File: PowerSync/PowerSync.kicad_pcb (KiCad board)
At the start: 2 copper layers, 107.3 x 48.9 mm, 40 parts, among them K12VDC1 G5RL-K1A-E, K9VAC1 G5RL-K1A-E, Q1 2N3904, Q2 2N3904, U1 74HCT1G04, U2 74HCT1G32, U3 74HCT74, U4 74HCT2G08

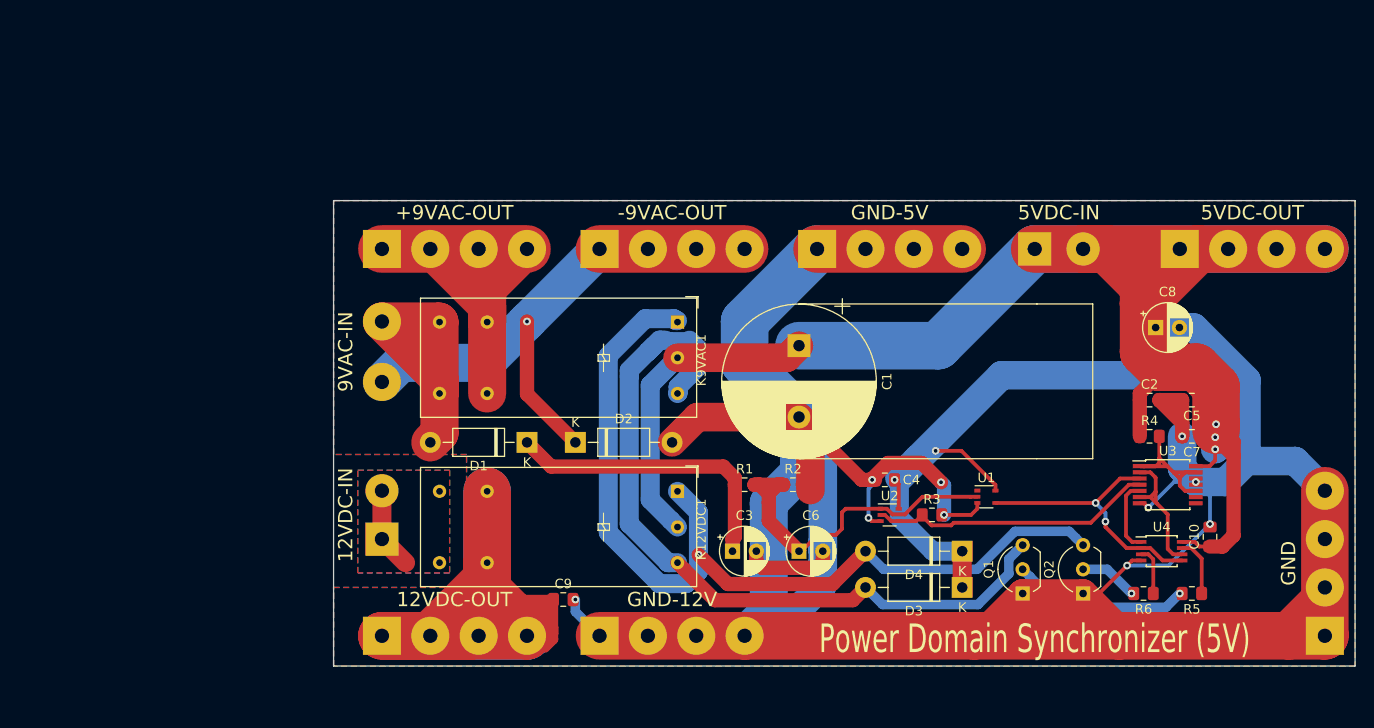
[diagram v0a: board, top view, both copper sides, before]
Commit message: Add files via upload
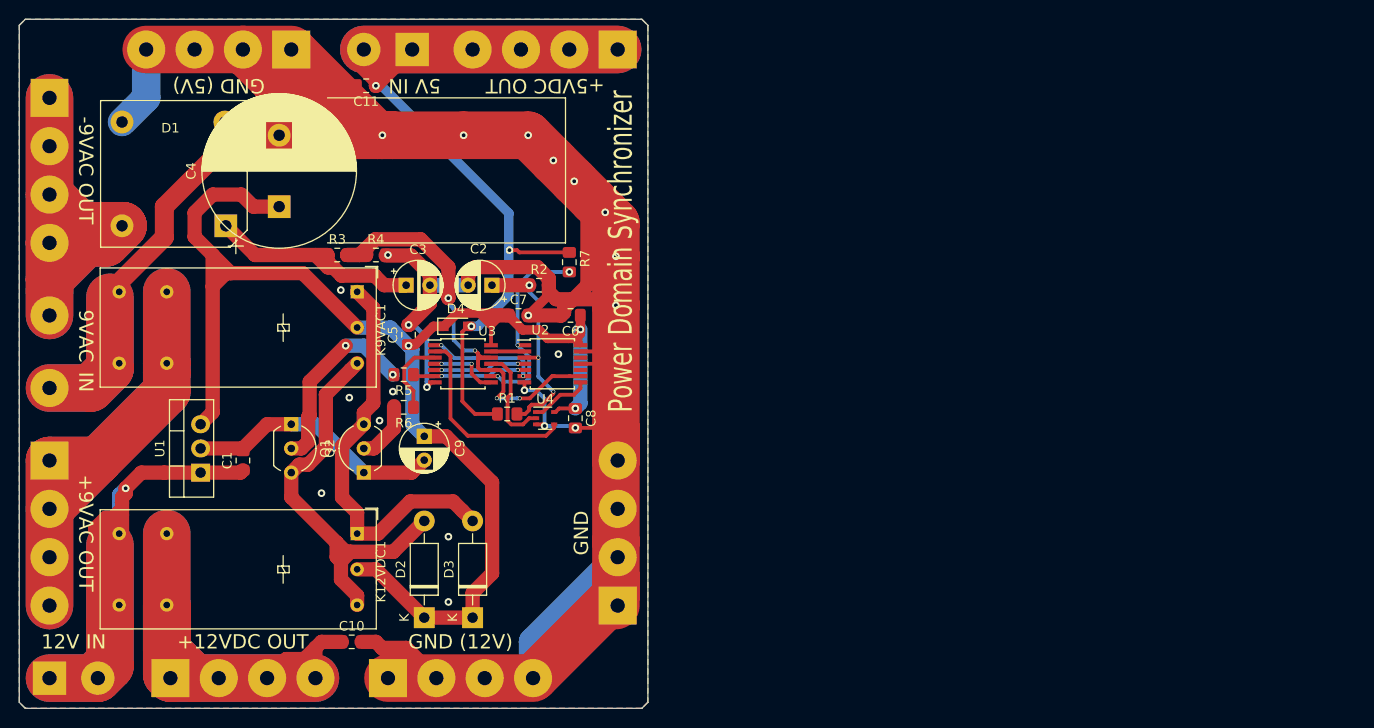
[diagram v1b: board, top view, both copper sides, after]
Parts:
- removed +9VAC-OUT, -9VAC-OUT, 12VDC-OUT, 5VDC-OUT, GND-12V: ~, Connector_Wire:SolderWirePad_1x04_P5.08mm_Drill1.5mm
- removed 12VDC-IN: +12VDC, Connector_Wire:SolderWirePad_1x02_P5.08mm_Drill1.5mm
- removed 5VDC-IN: +5VDC, Connector_Wire:SolderWirePad_1x02_P5.08mm_Drill1.5mm
- removed 9VAC-IN: +9VAC, Connector_Wire:SolderWirePad_1x01_Drill1.5mm
- removed GND-5V: GND, Connector_Wire:SolderWirePad_1x04_P5.08mm_Drill1.5mm
- removed IN-2: -9VAC, Connector_Wire:SolderWirePad_1x01_Drill1.5mm
- removed the REF** at (142.4, 83.1)
- added +12VDC OUT: ~, Connector_Wire:SolderWirePad_1x04_P5.08mm_Drill1.5mm, F.Cu at (58.4, 109.2)
- added +5VDC OUT: ~, Connector_Wire:SolderWirePad_1x04_P5.08mm_Drill1.5mm, F.Cu at (105.4, 43.2)
- added +9VAC OUT: ~, Connector_Wire:SolderWirePad_1x04_P5.08mm_Drill1.5mm, F.Cu at (45.7, 86.4)
- added -9VAC OUT: ~, Connector_Wire:SolderWirePad_1x04_P5.08mm_Drill1.5mm, F.Cu at (45.7, 48.3)
- added 12V IN: +12VDC, Connector_Wire:SolderWirePad_1x02_P5.08mm_Drill1.5mm, F.Cu at (45.7, 109.2)
- added 5V IN: +5VDC, Connector_Wire:SolderWirePad_1x02_P5.08mm_Drill1.5mm, F.Cu at (83.8, 43.2)
- added 9VAC: -9VAC, Connector_Wire:SolderWirePad_1x01_Drill1.5mm, F.Cu at (45.7, 71.1)
- added C11: 100n, Capacitor_SMD:C_0805_2012Metric_Pad1.15x1.40mm_HandSolder, F.Cu at (79.0, 47.0)
- added GND (12V): ~, Connector_Wire:SolderWirePad_1x04_P5.08mm_Drill1.5mm, F.Cu at (81.3, 109.2)
- added GND (5V): GND, Connector_Wire:SolderWirePad_1x04_P5.08mm_Drill1.5mm, F.Cu at (71.1, 43.2)
- added IN: +9VAC, Connector_Wire:SolderWirePad_1x01_Drill1.5mm, F.Cu at (45.7, 78.7)
- added R7: 220, Resistor_SMD:R_0805_2012Metric_Pad1.15x1.40mm_HandSolder, F.Cu at (100.3, 65.5)
- added REF**: OSHW-Logo_19x20mm_SilkScreen, Symbol:OSHW-Logo_19x20mm_SilkScreen, B.Cu at (92.8, 57.0)
- C1: value 10000u -> 220n; footprint Capacitor_THT:CP_Radial_D16.0mm_P7.50mm -> Capacitor_SMD:C_0805_2012Metric_Pad1.15x1.40mm_HandSolder
- C2: value 220n -> 1u; footprint Capacitor_SMD:C_0805_2012Metric_Pad1.15x1.40mm_HandSolder -> Capacitor_THT:CP_Radial_D5.0mm_P2.50mm
- C4: value 100n -> 10000u; footprint Capacitor_SMD:C_0805_2012Metric_Pad1.15x1.40mm_HandSolder -> Capacitor_THT:CP_Radial_D16.0mm_P7.50mm
- C5: value 47n -> 220n
- C6: value 2u2 -> 100n; footprint Capacitor_THT:CP_Radial_D5.0mm_P2.50mm -> Capacitor_SMD:C_0805_2012Metric_Pad1.15x1.40mm_HandSolder
- C7: value 10n -> 47n
- C8: value 10u -> 10n; footprint Capacitor_THT:CP_Radial_D5.0mm_P2.50mm -> Capacitor_SMD:C_0805_2012Metric_Pad1.15x1.40mm_HandSolder
- C9: value 100n -> 10u; footprint Capacitor_SMD:C_0805_2012Metric_Pad1.15x1.40mm_HandSolder -> Capacitor_THT:CP_Radial_D5.0mm_P2.50mm
- D1: value 1N4001 -> D_Bridge_+A-A; footprint Diode_THT:D_DO-41_SOD81_P10.16mm_Horizontal -> Diode_THT:Diode_Bridge_15.1x15.1x6.3mm_P10.9mm
- D4: value 1N4001 -> NSR0530HT1G; footprint Diode_THT:D_DO-41_SOD81_P10.16mm_Horizontal -> Diode_SMD:D_SOD-323_HandSoldering
- R1: value 33k -> 27k
- R2: value 20k -> 33k
- R3: value 8k2 -> 22k
- R4: value 8k2 -> 10k
- U1: value 74HCT1G04 -> LM7805_TO220; footprint Package_TO_SOT_SMD:SOT-353_SC-70-5 -> Package_TO_SOT_THT:TO-220-3_Vertical
- U2: value 74HCT1G32 -> 74HCT04; footprint Package_TO_SOT_SMD:SOT-353_SC-70-5 -> Package_SO:TSSOP-14_4.4x5mm_P0.65mm
- U3: value 74HCT74 -> 74HCT08
- U4: value 74HCT2G08 -> 74HCT1G32; footprint Package_SO:TSSOP-8_3x3mm_P0.65mm -> Package_TO_SOT_SMD:SOT-353_SC-70-5
- moved C10 90.8 mm to (77.5, 105.4), turned to 0 degrees
- moved R5 85.9 mm to (82.9, 77.3)
- moved R4 83.5 mm to (80.0, 64.8)
- moved U1 82.6 mm to (61.6, 87.6), turned to 90 degrees
- moved C5 82.6 mm to (83.4, 73.2), turned to 90 degrees
- moved R6 80.1 mm to (82.9, 80.8)
- moved Q1 78.9 mm to (71.1, 82.5), turned to 270 degrees
- moved Q2 76.6 mm to (78.7, 87.6)
- moved U3 75.1 mm to (89.2, 76.2)
- moved GND 74.4 mm to (105.4, 101.6)
- moved C7 71.9 mm to (95.0, 71.1), turned to 0 degrees
- moved C2 70.1 mm to (92.2, 67.9), turned to 180 degrees
- moved C4 69.8 mm to (69.8, 59.7), turned to 90 degrees
- moved R3 68.2 mm to (76.0, 64.8)
- moved U4 66.3 mm to (97.8, 81.9)
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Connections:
- C1 pad 1: +5V -> +12V
- C10 pad 1: +5V -> VDD
- C2 pad 1: +5V -> /TIMER-5V
- C4 pad 1: +5V -> VCC
- C5 pad 1: +5V -> VCC
- C6 pad 1: Net-(C6-Pad1) -> VCC
- C7 pad 1: +5V -> VCC
- C8 pad 1: +5V -> VCC
- C9 pad 1: VDD -> VCC
- D2 pad 1: NEUT -> VCC
- D2 pad 2: GND -> /~RELAY_SET
- D3 pad 1: +5V -> VCC
- D3 pad 2: /~RELAY_SET -> /~RELAY_RESET
- D4 pad 1: +5V -> VCC
- D4 pad 2: /~RELAY_RESET -> +5V
- K12VDC1 pad 9: +5V -> VCC
- K9VAC1 pad 9: +5V -> VCC
- R1 pad 1: Net-(C3-Pad1) -> +5V
- R1 pad 2: Net-(C6-Pad1) -> /TIMER-5V
- R2 pad 1: Net-(C6-Pad1) -> /TIMER-5V
- R3 pad 1: Net-(R3-Pad1) -> Net-(C3-Pad1)
- R3 pad 2: GND -> /DET_9VAC
- R4 pad 1: +5V -> /DET_9VAC
- R4 pad 2: /COMMON_PULLUP -> GND
- U1 pad 1: (no net) -> +12V
- U1 pad 2: Net-(C6-Pad1) -> GND
- U1 pad 3: GND -> VCC
- U2 pad 1: Net-(C6-Pad1) -> /DET_5V
- U2 pad 2: Net-(R3-Pad1) -> Net-(U2-Pad2)
- U2 pad 3: GND -> /TIMER-5V
- U2 pad 4: Net-(R3-Pad1) -> Net-(U2-Pad4)
- U2 pad 5: +5V -> Net-(R5-Pad1)
- U3 pad 1: /COMMON_PULLUP -> Net-(U2-Pad6)
- U3 pad 10: /COMMON_PULLUP -> /DET_9VAC
- U3 pad 11: GND -> Net-(U3-Pad11)
- U3 pad 12: GND -> /DET_9VAC
- U3 pad 13: /COMMON_PULLUP -> Net-(U2-Pad2)
- U3 pad 14: +5V -> VCC
- U3 pad 3: Net-(U1-Pad4) -> Net-(R6-Pad1)
- U3 pad 4: Net-(R3-Pad1) -> Net-(U3-Pad4)
- U3 pad 5: Net-(U3-Pad5) -> Net-(U2-Pad4)
- U3 pad 6: Net-(U3-Pad2) -> Net-(R5-Pad1)
- U3 pad 8: Net-(U3-Pad8) -> Net-(U3-Pad4)
- U3 pad 9: Net-(U3-Pad9) -> /DET_5V
- U4 pad 1: Net-(U3-Pad5) -> Net-(U2-Pad8)
- U4 pad 2: Net-(U1-Pad4) -> Net-(U3-Pad11)
- U4 pad 3: Net-(R6-Pad1) -> GND
- U4 pad 4: GND -> Net-(U3-Pad2)
- U4 pad 5: Net-(U1-Pad4) -> VCC
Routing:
- net +5V: track 280.5 -> 117.0 mm, vias 5 -> 3
- net VCC: track 0.00 -> 155.2 mm, vias 0 -> 3
- net +12V: track 8.59 -> 93.8 mm, vias 0 -> 1
- net /~RELAY_RESET: track 95.2 -> 42.5 mm, vias 1 -> 0
- net /DET_9VAC: track 0.00 -> 45.9 mm, vias 0 -> 4
- net VAC: track 50.6 -> 96.4 mm
- net NEUT: track 58.7 -> 100.9 mm, vias 1 -> 0
- net /~RELAY_SET: track 84.3 -> 44.0 mm
- net Net-(C6-Pad1): track 36.8 -> 0.00 mm
- net Net-(R3-Pad1): track 30.0 -> 0.00 mm
- net Net-(U1-Pad4): track 28.7 -> 0.00 mm, vias 2 -> 0
- net VDD: track 115.5 -> 91.6 mm
- net /TIMER-5V: track 0.00 -> 22.7 mm, vias 0 -> 3
- net +9VA: track 29.2 -> 51.9 mm
- net /DET_5V: track 0.00 -> 19.9 mm, vias 0 -> 3
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- removed copper zone on B.Cu, net +12V
- removed copper zone on F.Cu, net +12V
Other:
- board size 107.3 x 48.9 mm -> 66 x 72.4 mm
- board text added: "Commodore PowerSync"
- board text added: "Power Domain Synchronizer"
- board text removed: "Power Domain Synchronizer (5V)"
